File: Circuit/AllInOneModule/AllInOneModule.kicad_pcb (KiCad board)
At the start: 2 copper layers, 176.5 x 44.5 mm, 40 parts, among them J101 Servo, J102 KeyPad, Q3 DMG3415U, SW1 BOOT0, SW2 RESET, U1 ESP32-S3-MINI-1, U101 HT16K33, U2 AP2112/RT9080-3.3, U3 MCP73831T-2ACI/OT, X1 JSTPH, X3 USB C

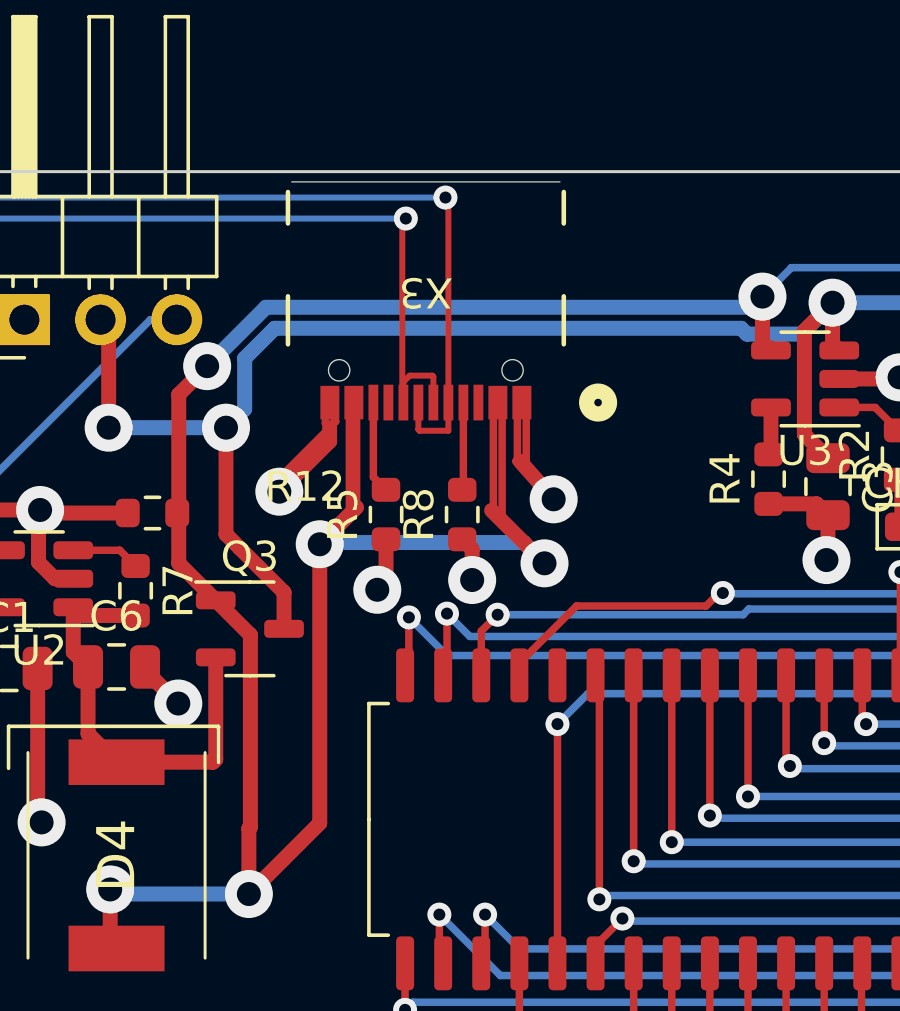
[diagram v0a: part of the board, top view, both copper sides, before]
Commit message: Snapshot commit.
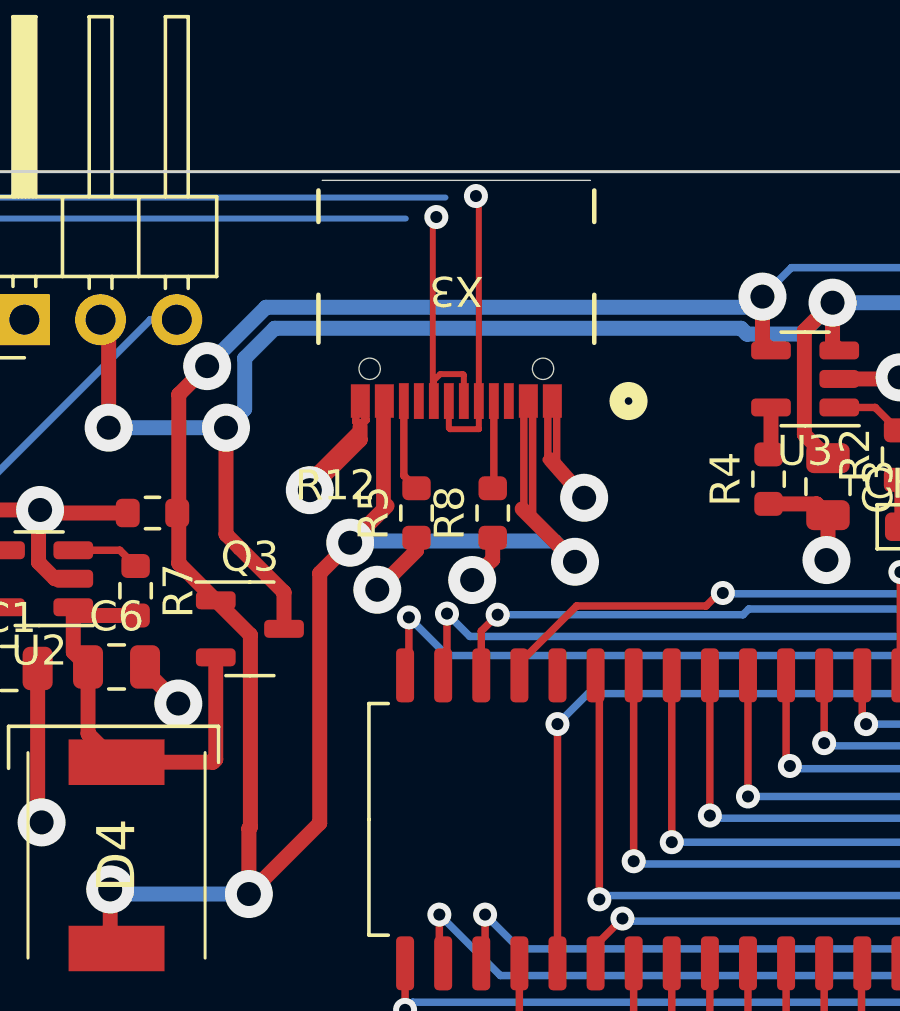
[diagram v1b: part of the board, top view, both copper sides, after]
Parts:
- moved X3 1.02 mm to (140.8, 35.7)
- moved R5 1.02 mm to (139.4, 43.1)
- moved R8 1.02 mm to (142.0, 43.1)
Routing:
- net GND: track 122.7 -> 123.4 mm

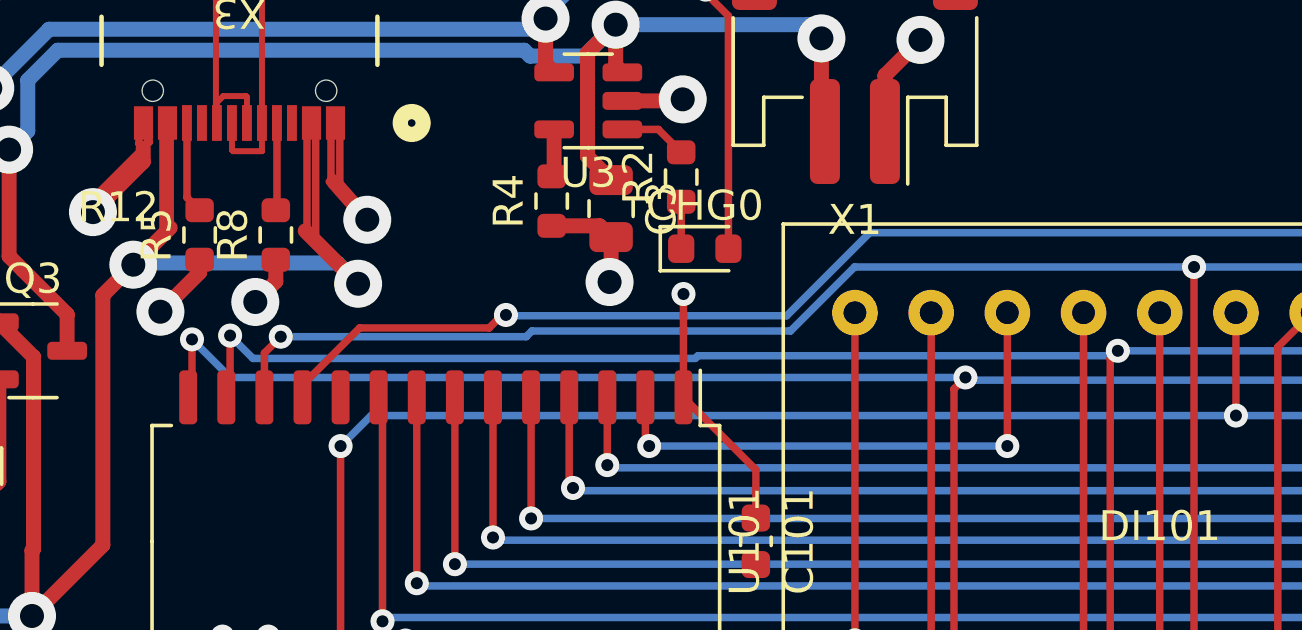
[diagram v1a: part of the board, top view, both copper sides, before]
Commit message: Snapshot commit.
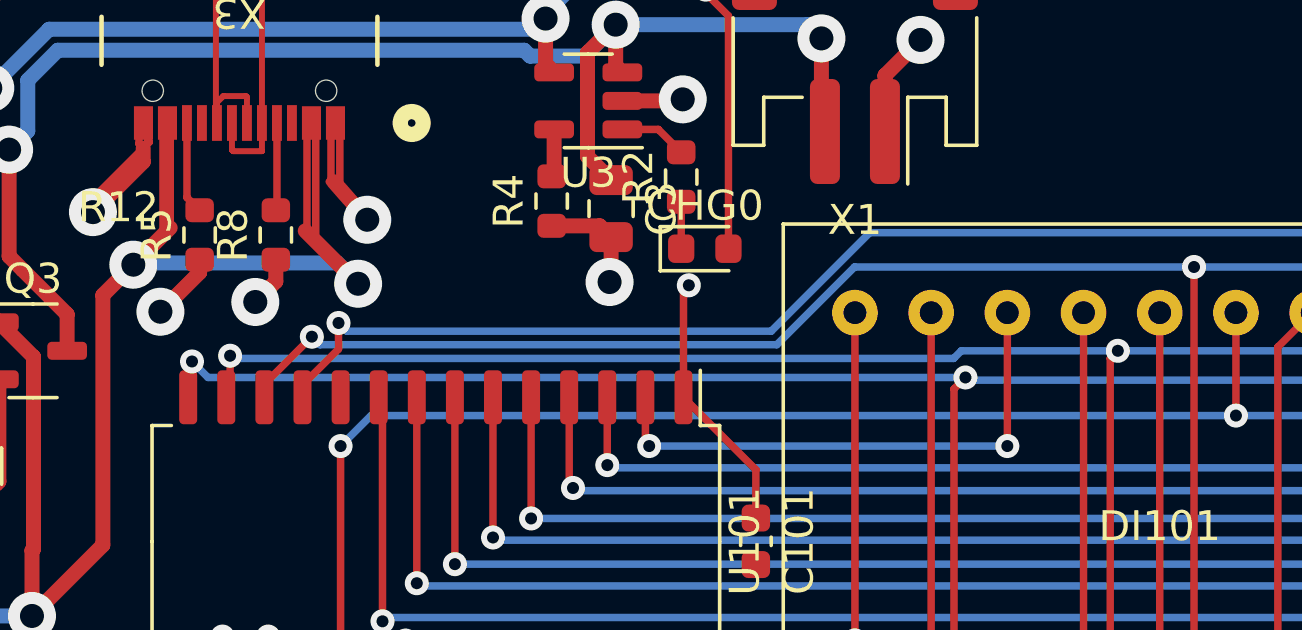
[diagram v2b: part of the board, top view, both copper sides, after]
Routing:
- net /Display Module/L: track 158.4 -> 157.4 mm
- net /Display Module/M: track 166.1 -> 165.1 mm
- net /Display Module/DP: track 187.6 -> 188.3 mm
